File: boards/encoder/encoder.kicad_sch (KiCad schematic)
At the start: 21 parts, among them SW1 SW_Push, SW2 SW_SPST, SW3 SW_SPST, U1 MSPM0G310x, U2 TPS62A02A, U3 TCAN1044V

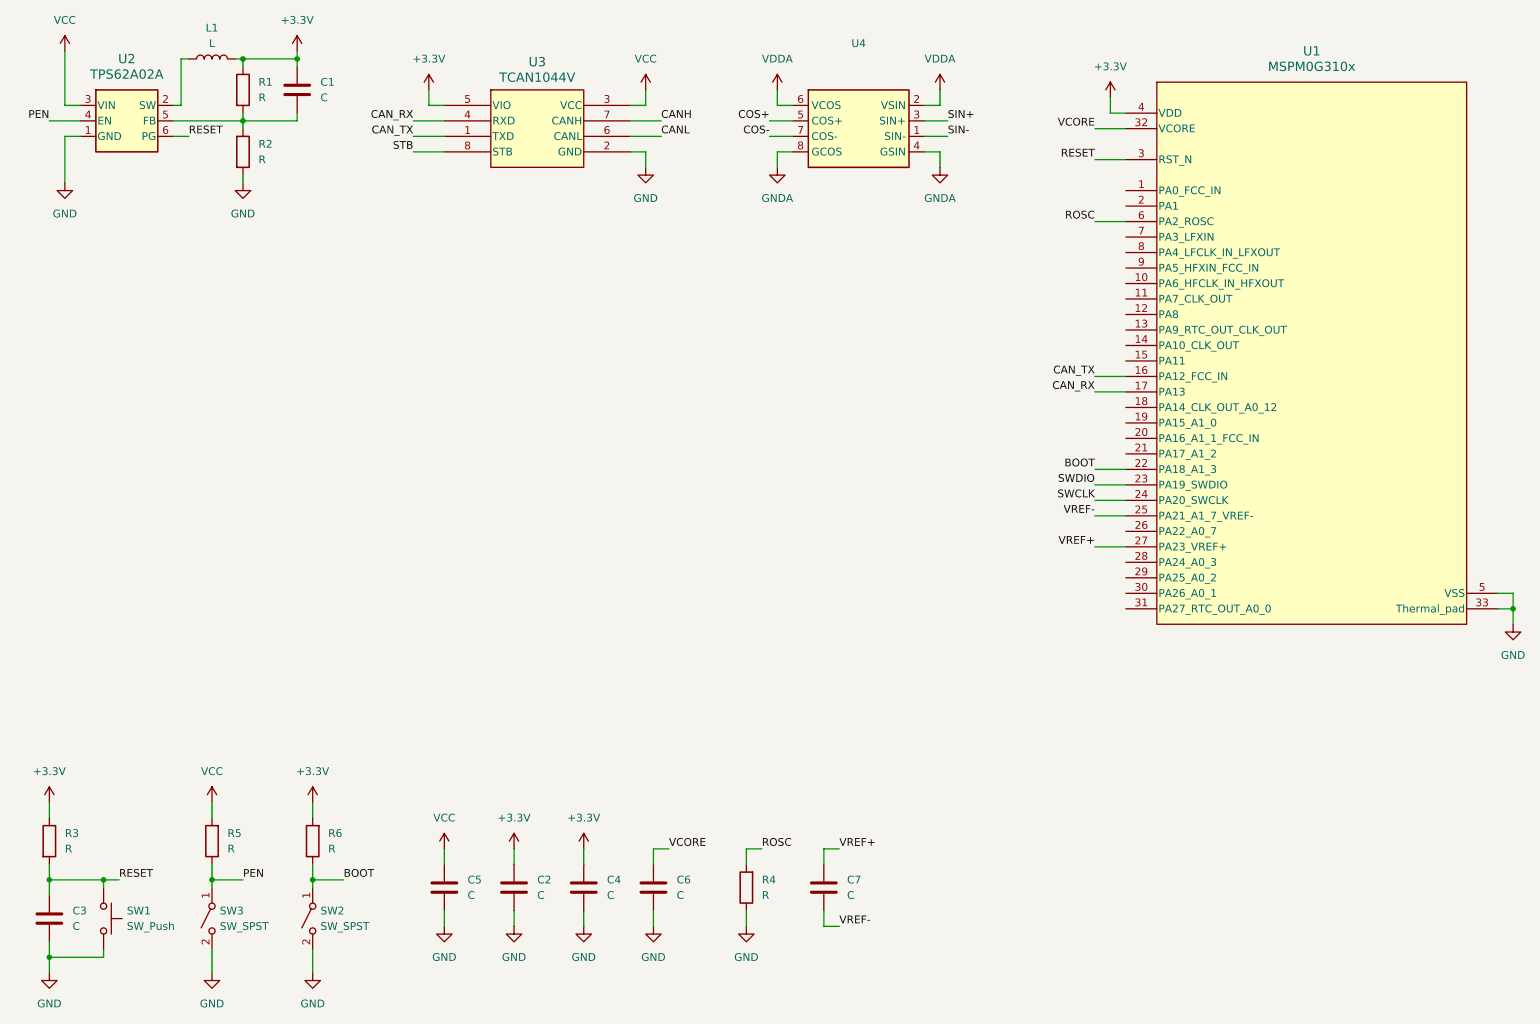
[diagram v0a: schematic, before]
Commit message: v0.1.3
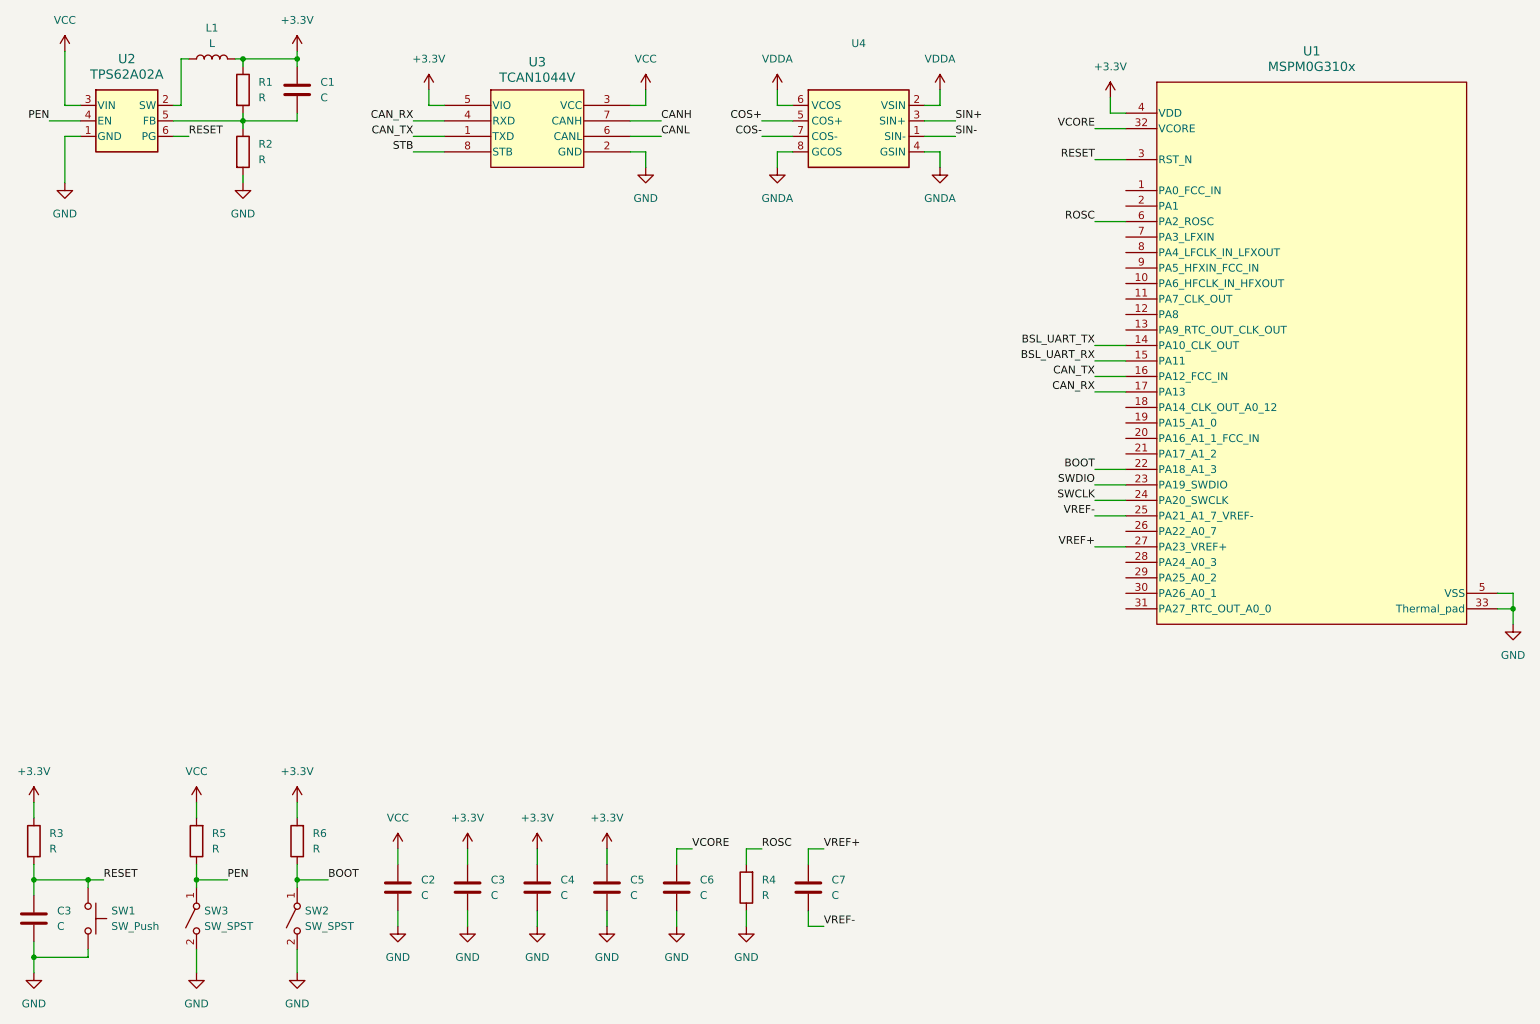
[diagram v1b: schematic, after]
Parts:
- added C5: C, symbol Device:C
- renumbered C5 to C2, C2 to C3
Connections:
- net +3.3V: now also C5.1
- net GND: now also C5.2
- net BSL_UART_TX: now reaches U1.14 (PA10_CLK_OUT)
- net BSL_UART_RX: now reaches U1.15 (PA11)
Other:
- moved on the sheet: C2, C3, C4, C6, C7, R3, R5, R6, SW1, SW2, SW3
